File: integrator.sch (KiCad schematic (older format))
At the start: 94 parts, among them J1 SJ-3524-SMT, J2 SJ-3524-SMT, J3 SP-3533-02, J4 SP-3533-02, J5 USB4105-GF-A, J6 Conn_ARM_JTAG_SWD_10, J7 test point, SW1 EVQP40B3M, SW2 EVQP40B3M, SW3 EVQP40B3M, SW4 436333033816, U1 XC6415, U2 MCP1700-2302E/TT, U3 LSM6DSO32XTR, U4 NL27WZ16DTT1G, U5 RP2040, U6 IS25WP128F-JBLE, U7 NL27WZ16DTT1G, Y1 Crystal

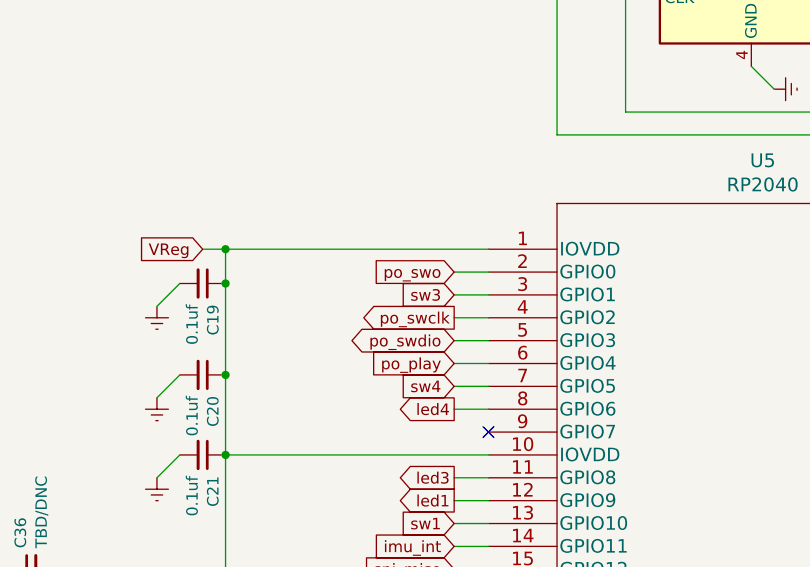
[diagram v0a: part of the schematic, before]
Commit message: moved logos, misc tweaks
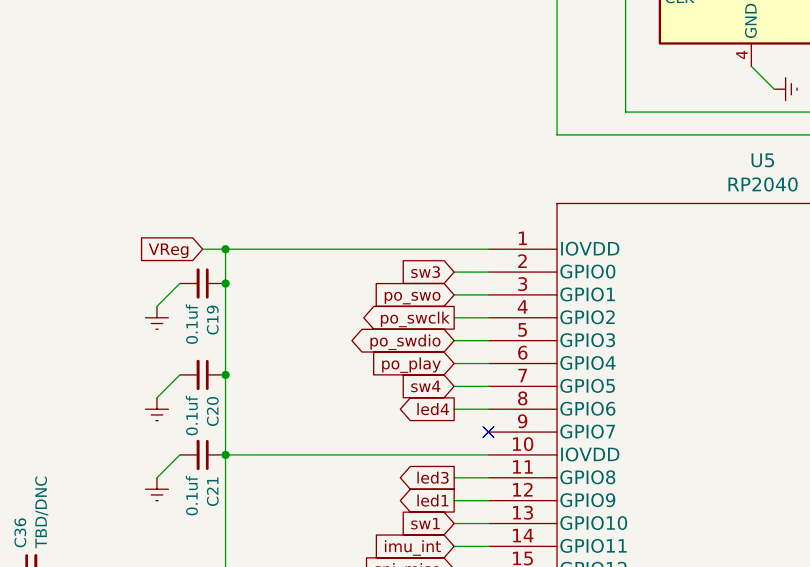
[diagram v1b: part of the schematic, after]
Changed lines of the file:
@@
 Text GLabel 9900 6950 2    50   Input ~ 0
 sw2
-Text GLabel 7250 5050 0    50   Input ~ 0
+Text GLabel 7250 4950 0    50   Input ~ 0
 sw3
 Text GLabel 7250 5450 0    50   Input ~ 0
@@
 Text GLabel 7250 5250 0    50   BiDi ~ 0
 po_swdio
-Text GLabel 7250 4950 0    50   Input ~ 0
+Text GLabel 7250 5050 0    50   Input ~ 0
 po_swo
 Text GLabel 7250 5350 0    50   Input ~ 0
